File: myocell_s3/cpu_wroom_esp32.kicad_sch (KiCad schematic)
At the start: 16 parts, among them SW1 SW_Push, SW2 SW_Push, U4 ESP32-WROOM-E

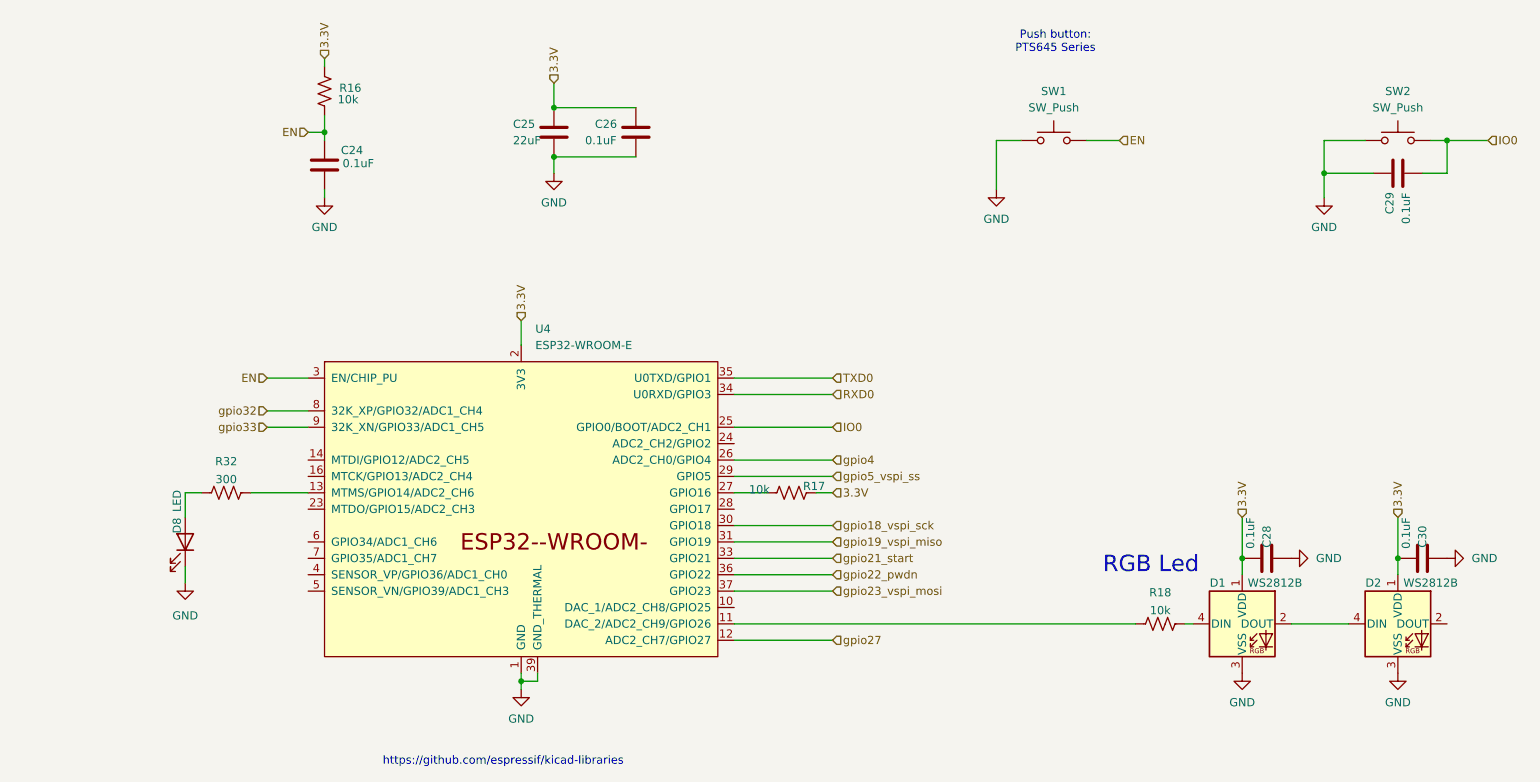
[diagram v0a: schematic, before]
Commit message: recovery commit
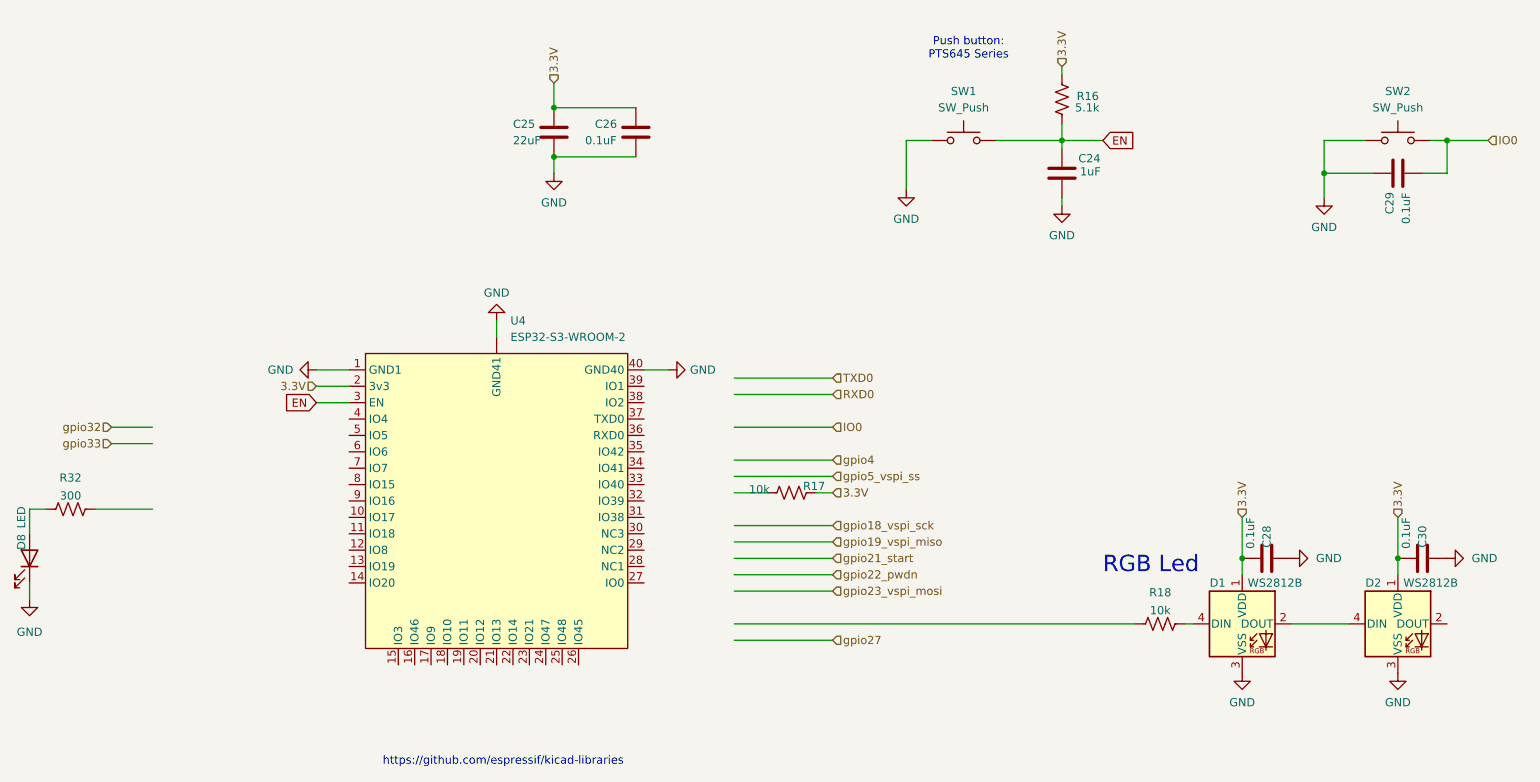
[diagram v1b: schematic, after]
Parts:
- removed U4: ESP32-WROOM-E, RF_Module:ESP32-WROOM-32E, symbol espressif_github:ESP32-WROOM-E
- added U4: ESP32-S3-WROOM-2, RF_Module:ESP32-S3-WROOM-2, symbol myocell_s3:ESP32-S3-WROOM-2
- C24: value 0.1uF -> 1uF
- R16: value 10k -> 5.1k
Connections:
- net 3.3V: now also U4.2 (3v3)
- net EN: now also U4.3 (EN)
- net GND: now also U4. (GND41), U4.1 (GND1), U4.40 (GND40)
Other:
- moved on the sheet: C24, D8, R16, R32, SW1
